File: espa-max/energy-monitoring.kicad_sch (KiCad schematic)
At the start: 5 parts, among them J5 AudioPlug2

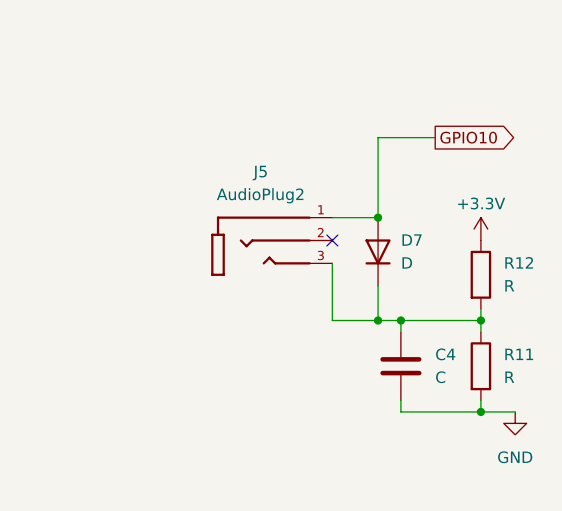
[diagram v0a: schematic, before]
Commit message: Misc updates from a while back. Committing before I do an update to use smaller components.
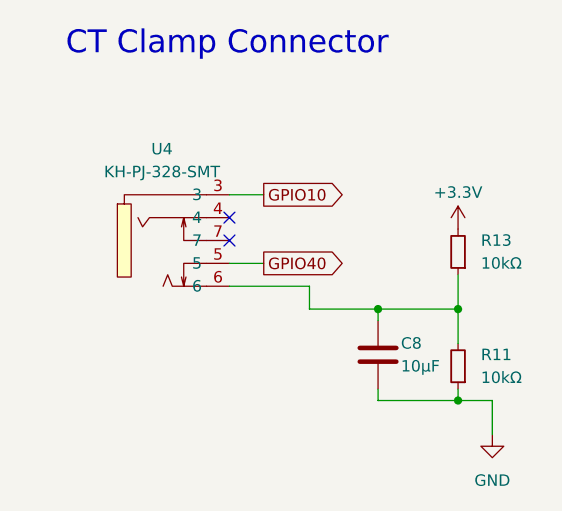
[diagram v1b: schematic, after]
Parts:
- removed C4: C, symbol Device:C
- removed D7: D, symbol Device:D
- removed J5: AudioPlug2, PJ-320B:BOOMELE_PJ-320B, symbol PJ-320B:PJ-320B
- removed R11, R12: R, symbol Device:R
- added C8: 10μF, Capacitor_SMD:C_0603_1608Metric, symbol Device:C
- added R11, R13: 10kΩ, Resistor_SMD:R_0603_1608Metric, symbol Device:R_Small
- added U4: KH-PJ-328-SMT, 3.5mm-connector:AUDIO-SMD_KH-PJ-328-SMT, symbol 3.5mm-connector:KH-PJ-328-SMT
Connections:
- net +3.3V: now also R13.2
- net GND: now also C8.2, R11.1
- net GPIO10: now also U4.3
- new net: C8.1, R11.2, R13.1, U4.6
- new net GPIO40: U4.5
- no-connect marks 1 -> 2
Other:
- note added: "CT Clamp Connector"
